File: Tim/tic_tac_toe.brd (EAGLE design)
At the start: 53.3 x 52.7 mm, 18 parts, among them IC1 PCF8574P, U1 ATMEGA328P_PDIP

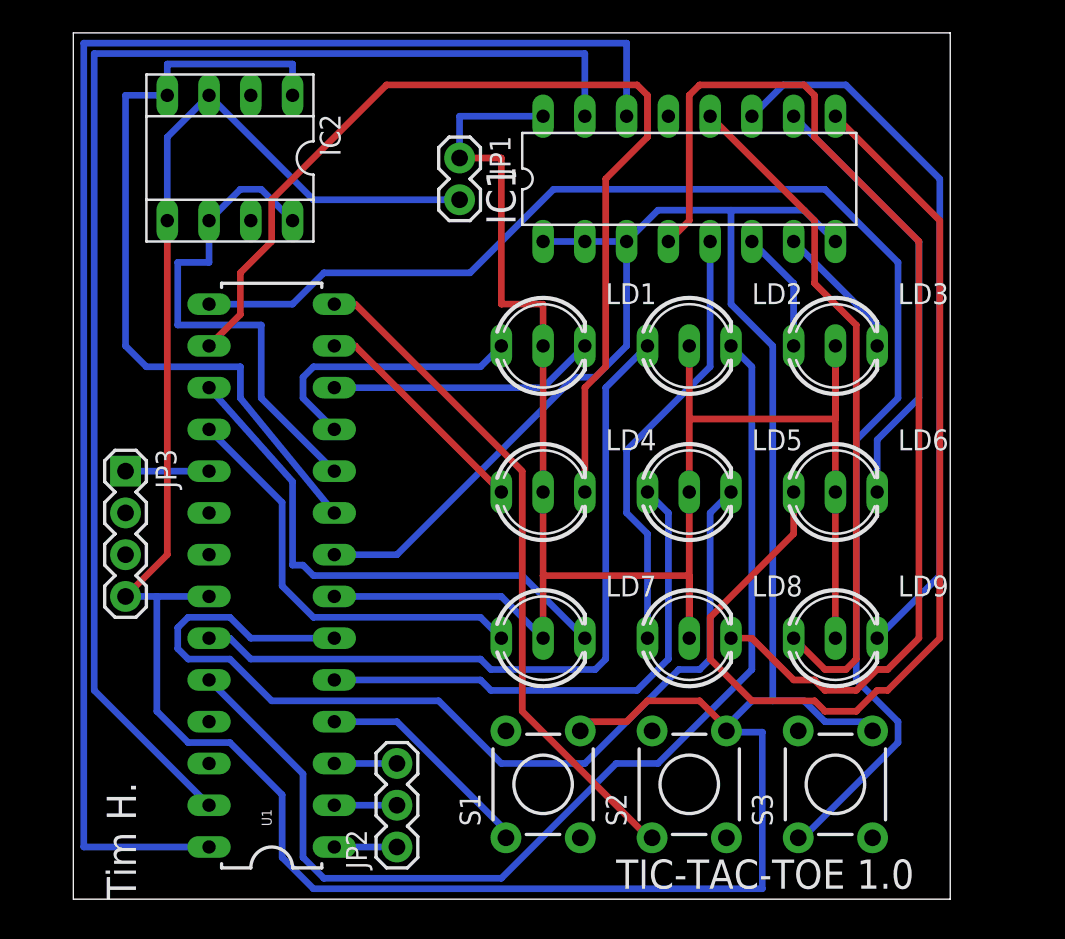
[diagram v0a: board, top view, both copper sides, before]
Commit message: 3 try
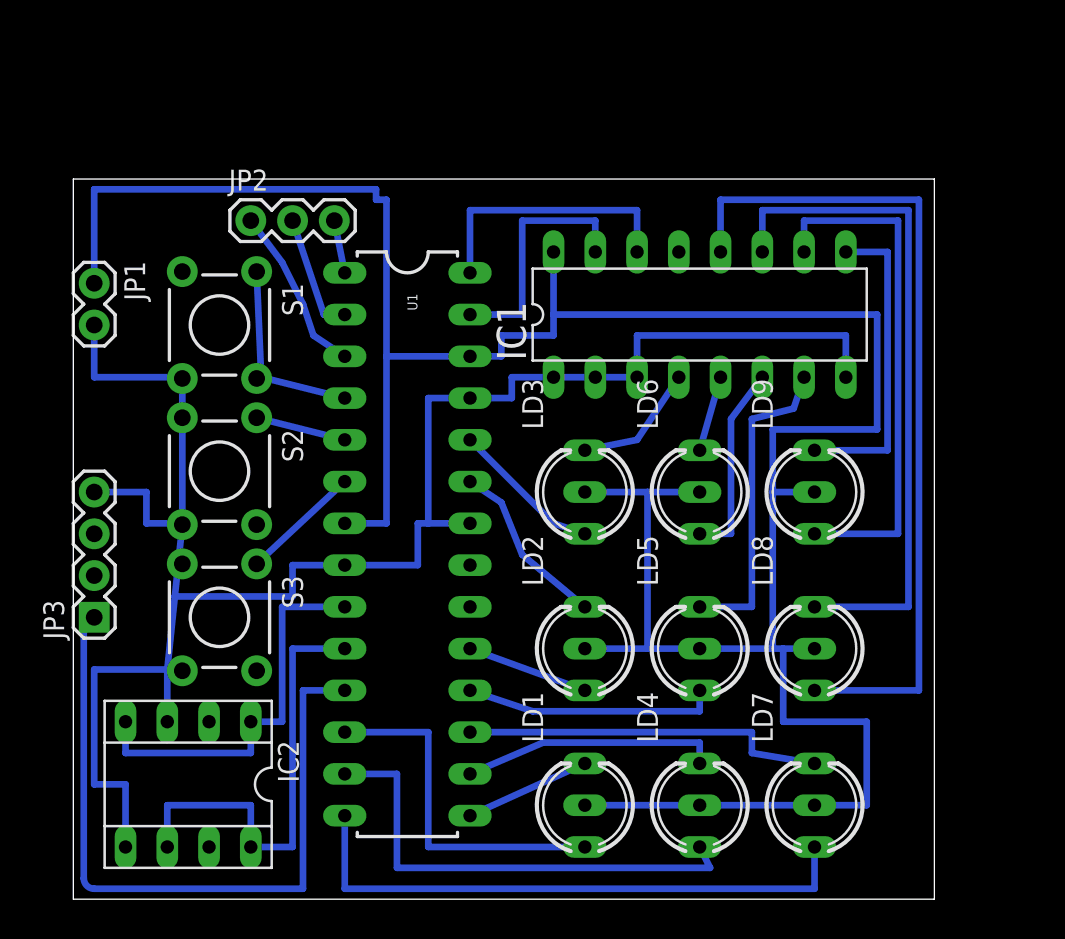
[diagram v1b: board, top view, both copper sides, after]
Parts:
- moved JP2 39.1 mm to (10.8, 41.3), turned to 0 degrees
- moved S3 38.8 mm to (8.89, 17.1), turned to 270 degrees
- moved IC2 38.2 mm to (6.99, 6.99)
- moved S2 34.3 mm to (8.89, 26.0), turned to 270 degrees
- moved S1 34.2 mm to (8.89, 34.9), turned to 270 degrees
- moved LD1 28.1 mm to (31.1, 5.71), turned to 90 degrees
- moved JP1 23.5 mm to (1.27, 37.5)
- moved LD4 21.3 mm to (38.1, 5.71), turned to 90 degrees
- moved LD2 19.5 mm to (31.1, 15.2), turned to 90 degrees
- moved LD7 19.4 mm to (45.1, 5.71), turned to 90 degrees
- moved LD3 17.6 mm to (31.1, 24.8), turned to 90 degrees
- moved LD5 9.55 mm to (38.1, 15.2), turned to 90 degrees
- moved JP3 9.09 mm to (1.27, 17.1), turned to 90 degrees
- moved LD9 8.98 mm to (45.1, 24.8), turned to 90 degrees
- moved U1 8.47 mm to (20.3, 21.6), turned to 270 degrees
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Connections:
- net N$24 renamed S$6
- net N$25 renamed S$5
- net N$26 renamed S$2
- removed net N$10: JP3.1, U1.19
- removed net N$15: IC1.12, LD9.AX
- removed net N$16: IC1.11, LD9.AR
- removed net N$17: IC1.10, LD6.AR
- removed net N$18: IC1.9, LD6.AX
- removed net N$19: IC1.7, LD3.AR
- removed net N$20: IC1.6, LD3.AX
- removed net N$21: IC1.5, LD8.AX
- removed net N$22: IC1.4, LD8.AR
- removed net N$23: LD7.AX, U1.18
- removed net N$27: LD1.AR, U1.12
- removed net N$28: LD1.AX, U1.11
- removed net N$29: LD5.AR, U1.6
- removed net N$30: LD5.AX, U1.5
- removed net N$31: LD2.AX, U1.23
- removed net N$32: LD2.AR, U1.24
- removed net N$7 (its old number): JP2.1, U1.1
- new net N$6: JP3.1, U1.11
- new net N$9: JP2.3, U1.1
- new net S$1: LD1.AX, U1.12
- new net S$10: LD3.AX, U1.24
- new net S$11: IC1.4, LD3.AR
- new net S$12: IC1.5, LD6.AR
- new net S$13: IC1.6, LD6.AX
- new net S$14: IC1.7, LD5.AR
- new net S$15: IC1.9, LD9.AR
- new net S$16: IC1.10, LD9.AX
- new net S$17: IC1.11, LD8.AR
- new net S$18: IC1.12, LD8.AX
- new net S$3: LD7.AX, U1.14
- new net S$4: LD1.AR, U1.15
- new net S$7: LD5.AX, U1.18
- new net S$8: LD2.AX, U1.19
- new net S$9: LD2.AR, U1.23
- net N$2: now also U1.5; no longer U1.14
- net N$3: now also U1.6; no longer U1.15
- net N$8: now also JP2.1; no longer JP2.3
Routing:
- net GND: track 219.0 -> 117.4 mm
- net N$3: track 86.4 -> 7.33 mm
- net N$4: track 94.0 -> 16.5 mm
- net N$22: track 67.3 -> 0.00 mm
- net N$5: track 82.3 -> 15.2 mm
- net N$32: track 66.5 -> 0.00 mm
- net N$18: track 63.8 -> 0.00 mm
- net N$29: track 60.2 -> 0.00 mm
- net VCC: track 117.3 -> 174.0 mm
- net S$18: track 0.00 -> 51.4 mm
- net S$5: track 62.2 -> 15.6 mm
- net N$31: track 45.3 -> 0.00 mm
- net N$6: track 0.00 -> 44.3 mm
- net N$16: track 44.1 -> 0.00 mm
- net N$15: track 41.6 -> 0.00 mm
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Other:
- board size 53.3 x 52.7 mm -> 52.4 x 43.8 mm
- board text removed: "TIC-TAC-TOE 1.0"
- board text removed: "Tim H."
